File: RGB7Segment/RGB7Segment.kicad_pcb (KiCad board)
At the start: 2 copper layers, 30 parts, among them J1 Conn_01x02_Socket, J2 Conn_01x04_Pin

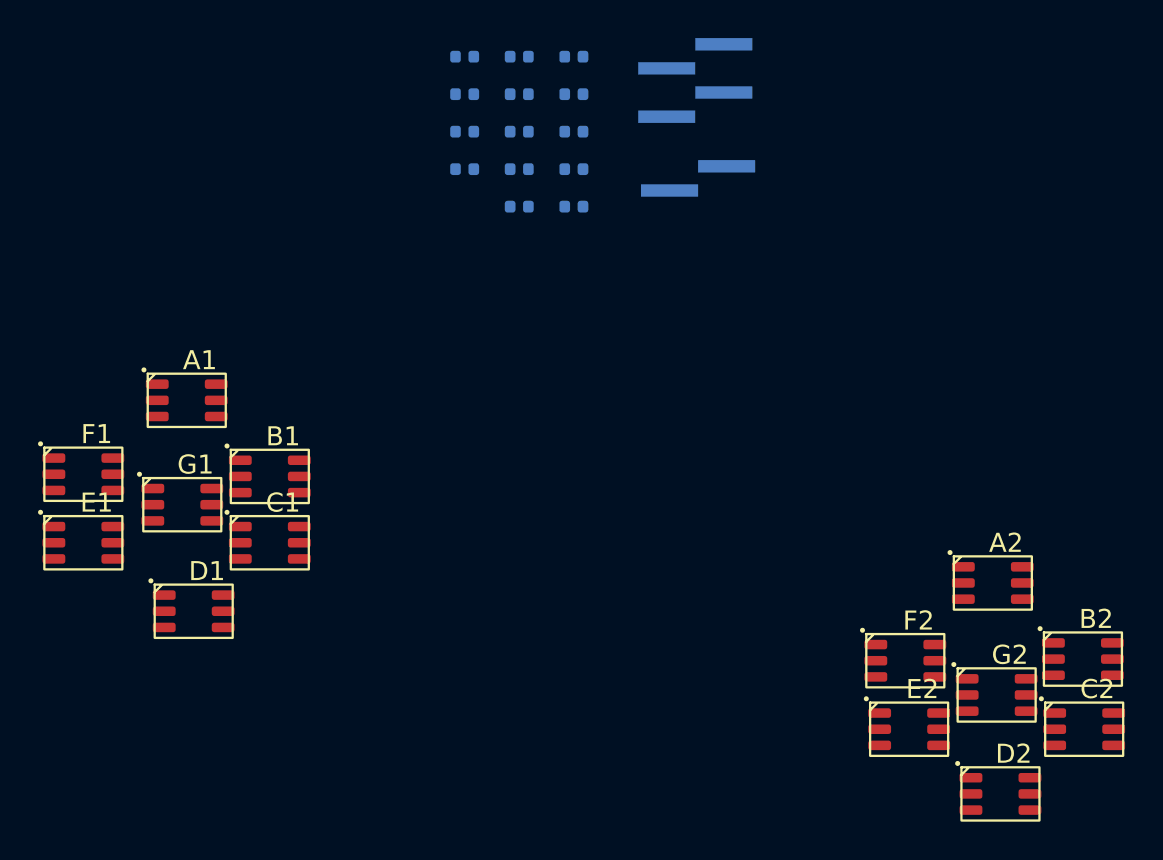
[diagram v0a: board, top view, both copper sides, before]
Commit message: Adding Project Setup
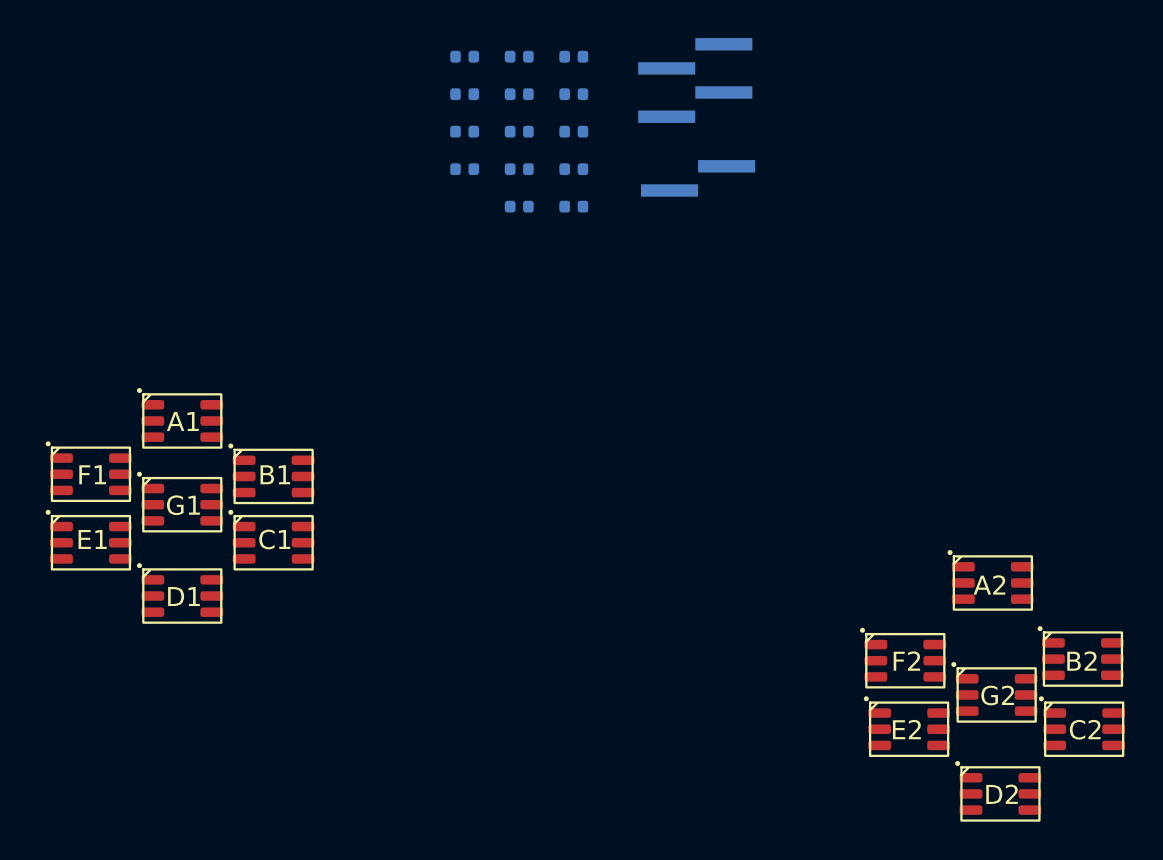
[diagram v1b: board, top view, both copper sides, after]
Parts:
- moved A1 1.11 mm to (225.4, 101.1)
- moved D1 1.00 mm to (225.4, 110.3)
- moved E1 0.40 mm to (220.6, 107.5)
- moved F1 0.40 mm to (220.6, 103.9)
- moved B1 0.20 mm to (230.2, 104.0)
- moved C1 0.20 mm to (230.2, 107.5)
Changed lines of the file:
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@@
 		(at 225.365356 105.485356)
 		(property "Reference" "G1"
-			(at 2.25 -1.25 0)
+			(at 1.634644 0.914644 0)
 			(unlocked yes)
 			(layer "F.SilkS")
@@
 		(at 267.965356 109.6)
 		(property "Reference" "A2"
-			(at 2.25 -1.25 0)
+			(at 1.434644 1 0)
 			(unlocked yes)
 			(layer "F.SilkS")
@@
 	(footprint "Library:587-2086-247F"
 		(layer "F.Cu")
-		(at 229.965356 104)
+		(at 230.165356 104)
 		(property "Reference" "B1"
-			(at 2.25 -1.25 0)
+			(at 1.634644 0.8 0)
 			(unlocked yes)
 			(layer "F.SilkS")
@@
 		(at 272.765356 117.285356)
 		(property "Reference" "C2"
-			(at 2.25 -1.25 0)
+			(at 1.634644 0.914644 0)
 			(unlocked yes)
 			(layer "F.SilkS")
@@
 		(at 272.7 113.6)
 		(property "Reference" "B2"
-			(at 2.25 -1.25 0)
+			(at 1.5 1 0)
 			(unlocked yes)
 			(layer "F.SilkS")
@@
 		(at 263.565356 117.285356)
 		(property "Reference" "E2"
-			(at 2.25 -1.25 0)
+			(at 1.434644 0.914644 0)
 			(unlocked yes)
 			(layer "F.SilkS")
@@
 		(at 268.165356 115.485356)
 		(property "Reference" "G2"
-			(at 2.25 -1.25 0)
+			(at 1.634644 0.914644 0)
 			(unlocked yes)
 			(layer "F.SilkS")
@@
 	(footprint "Library:587-2086-247F"
 		(layer "F.Cu")
-		(at 229.965356 107.485356)
+		(at 230.165356 107.485356)
 		(property "Reference" "C1"
-			(at 2.25 -1.25 0)
+			(at 1.634644 0.714644 0)
 			(unlocked yes)
 			(layer "F.SilkS")
@@
 	(footprint "Library:587-2086-247F"
 		(layer "F.Cu")
-		(at 225.6 100)
+		(at 225.365356 101.085356)
 		(property "Reference" "A1"
-			(at 2.25 -1.25 0)
+			(at 1.634644 0.914644 0)
 			(unlocked yes)
 			(layer "F.SilkS")
@@
 	(footprint "Library:587-2086-247F"
 		(layer "F.Cu")
-		(at 220.165356 107.485356)
+		(at 220.565356 107.485356)
 		(property "Reference" "E1"
-			(at 2.25 -1.25 0)
+			(at 1.634644 0.714644 0)
 			(unlocked yes)
 			(layer "F.SilkS")
@@
 	(footprint "Library:587-2086-247F"
 		(layer "F.Cu")
-		(at 220.165356 103.885356)
+		(at 220.565356 103.885356)
 		(property "Reference" "F1"
-			(at 2.25 -1.25 0)
+			(at 1.634644 0.914644 0)
 			(unlocked yes)
 			(layer "F.SilkS")
@@
 	(footprint "Library:587-2086-247F"
 		(layer "F.Cu")
-		(at 225.965356 111.085356)
+		(at 225.365356 110.285356)
 		(property "Reference" "D1"
-			(at 2.25 -1.25 0)
+			(at 1.634644 0.914644 0)
 			(unlocked yes)
 			(layer "F.SilkS")
@@
 		(at 263.365356 113.685356)
 		(property "Reference" "F2"
-			(at 2.25 -1.25 0)
+			(at 1.634644 0.914644 0)
 			(unlocked yes)
 			(layer "F.SilkS")
@@
 		(at 268.365356 120.685356)
 		(property "Reference" "D2"
-			(at 2.25 -1.25 0)
-			(unlocked yes)
-			(layer "F.SilkS")
+			(at 1.634644 0.914644 0)
+			(unlocked yes)
+			(layer "F.SilkS")

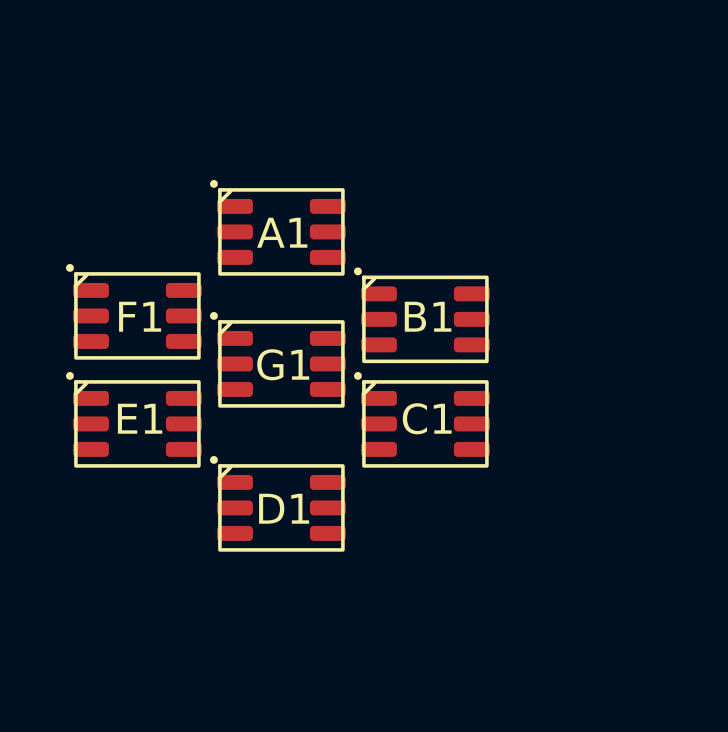
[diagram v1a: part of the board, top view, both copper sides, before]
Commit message: Standard push of SW in progress
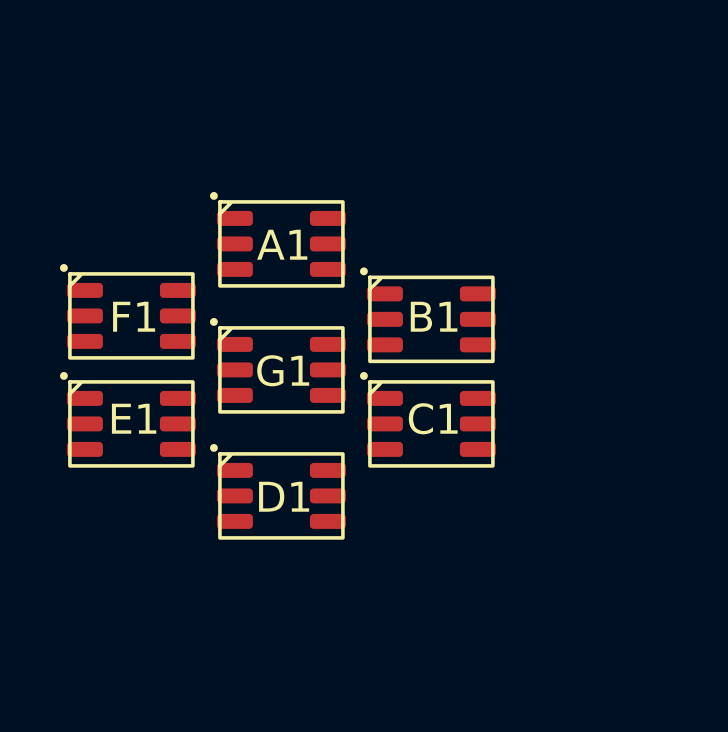
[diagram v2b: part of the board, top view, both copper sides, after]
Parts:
- moved A1 0.40 mm to (225.4, 101.5)
- moved D1 0.40 mm to (225.4, 109.9)
- moved E1 0.20 mm to (220.4, 107.5)
- moved F1 0.20 mm to (220.4, 103.9)
- moved G1 0.20 mm to (225.4, 105.7)
- moved B1 0.20 mm to (230.4, 104.0)
- moved C1 0.20 mm to (230.4, 107.5)
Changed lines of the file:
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@@
 	(footprint "Library:587-2086-247F"
 		(layer "F.Cu")
-		(at 225.365356 105.485356)
+		(at 225.365356 105.685356)
 		(property "Reference" "G1"
 			(at 1.634644 0.914644 0)
@@
 	(footprint "Library:587-2086-247F"
 		(layer "F.Cu")
-		(at 230.165356 104)
+		(at 230.365356 104)
 		(property "Reference" "B1"
 			(at 1.634644 0.8 0)
@@
 	(footprint "Library:587-2086-247F"
 		(layer "F.Cu")
-		(at 230.165356 107.485356)
+		(at 230.365356 107.485356)
 		(property "Reference" "C1"
 			(at 1.634644 0.714644 0)
@@
 	(footprint "Library:587-2086-247F"
 		(layer "F.Cu")
-		(at 225.365356 101.085356)
+		(at 225.365356 101.485356)
 		(property "Reference" "A1"
 			(at 1.634644 0.914644 0)
@@
 	(footprint "Library:587-2086-247F"
 		(layer "F.Cu")
-		(at 220.565356 107.485356)
+		(at 220.365356 107.485356)
 		(property "Reference" "E1"
 			(at 1.634644 0.714644 0)
@@
 	(footprint "Library:587-2086-247F"
 		(layer "F.Cu")
-		(at 220.565356 103.885356)
+		(at 220.365356 103.885356)
 		(property "Reference" "F1"
 			(at 1.634644 0.914644 0)
@@
 	(footprint "Library:587-2086-247F"
 		(layer "F.Cu")
-		(at 225.365356 110.285356)
+		(at 225.365356 109.885356)
 		(property "Reference" "D1"
 			(at 1.634644 0.914644 0)
